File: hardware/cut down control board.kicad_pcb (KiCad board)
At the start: 2 copper layers, 42 parts, among them J1 CUTTER, J10 SAT(10 picoblade), J11 VGPS SELECT, J2 MOTOR, J3 AVR-ISP-6, J5 SAT(PIN HDR), J6 GPS(PIN HDR), J7 DBG TTL, J9 GPS(JST SH), Q1 FQP30N06L, Q2 FQP30N06L, U1 ATmega328-P, U2 MPL3115A2, U5 L78L33_TO92, U6 L7805, Y1 16MHz

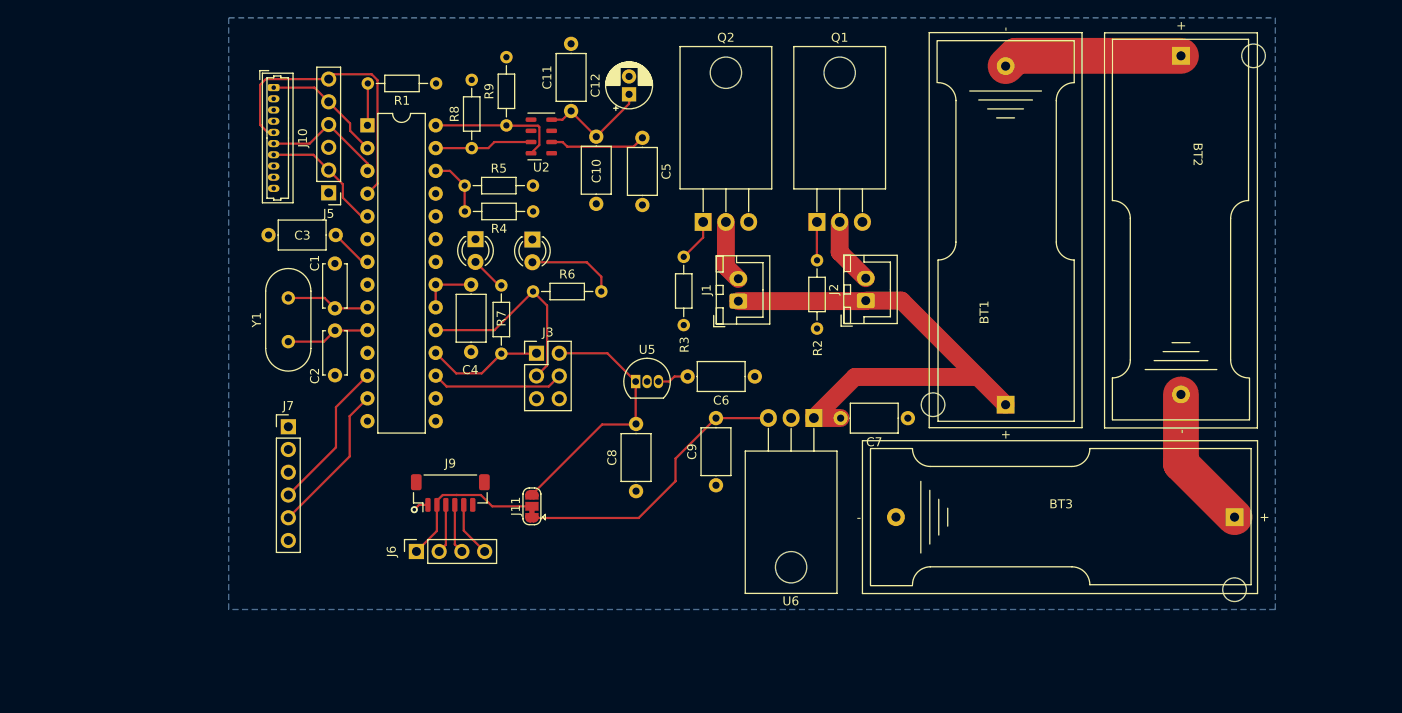
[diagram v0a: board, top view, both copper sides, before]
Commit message: finished board, generated gerbers
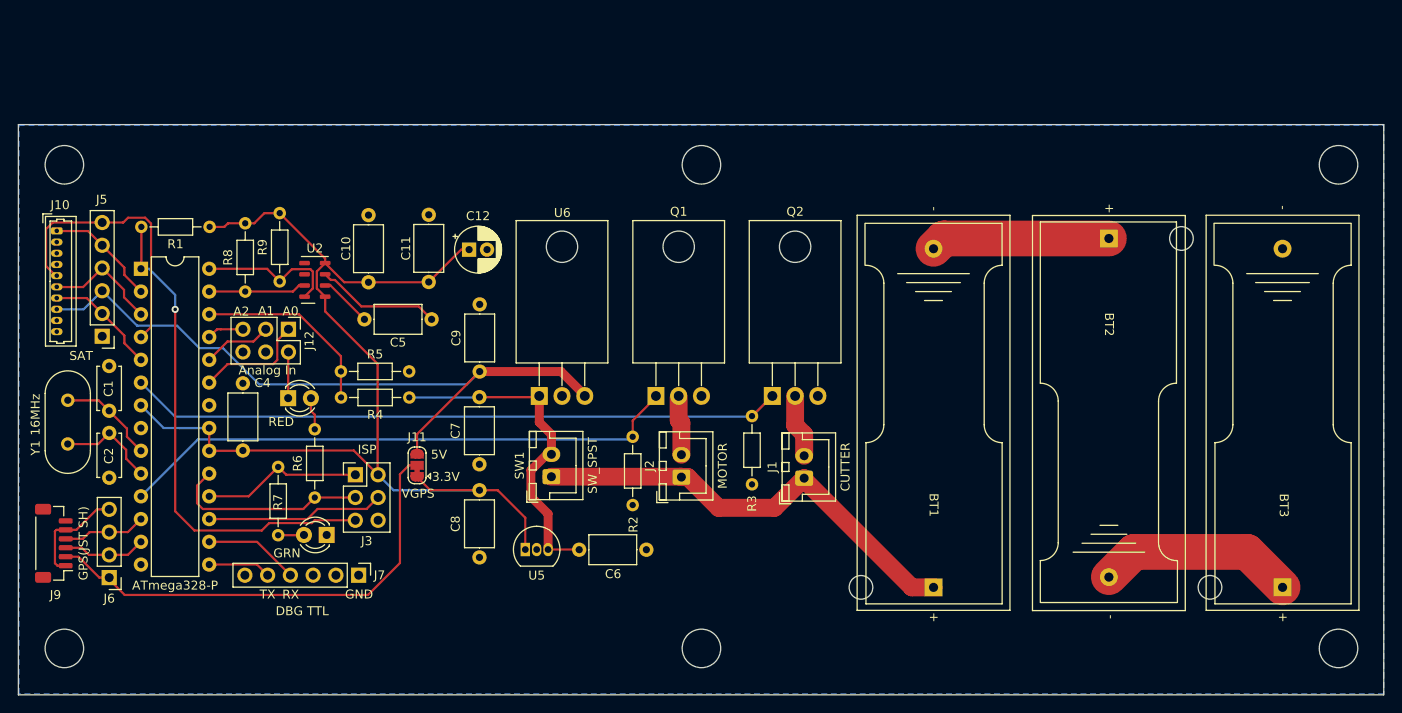
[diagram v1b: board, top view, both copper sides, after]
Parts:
- removed C3: 100nF, Capacitor_THT:C_Axial_L5.1mm_D3.1mm_P7.50mm_Horizontal
- added ?: , , F.Cu at (151.8, 126.3)
- added ?: , , F.Cu at (80.7, 72.3)
- added ?: , , F.Cu at (80.7, 126.3)
- added ?: , , F.Cu at (151.8, 72.3)
- added ?: , , F.Cu at (223.0, 126.3)
- added ?: , , F.Cu at (223.0, 72.3)
- added J12: Analog In, Connector_PinHeader_2.54mm:PinHeader_2x03_P2.54mm_Vertical, F.Cu at (105.7, 90.6)
- added SW1: SW_SPST, Connector_JST:JST_XH_B2B-XH-A_1x02_P2.50mm_Vertical, F.Cu at (135.1, 107.1)
- J3: value AVR-ISP-6 -> ISP
- J6: footprint Connector_PinSocket_2.54mm:PinSocket_1x04_P2.54mm_Vertical -> Connector_PinHeader_2.54mm:PinHeader_1x04_P2.54mm_Vertical
- moved C7 48.1 mm to (127.1, 105.7), turned to 90 degrees
- moved J9 44.6 mm to (79.5, 114.5), turned to 90 degrees
- moved C5 37.1 mm to (114.2, 89.5), turned to 0 degrees
- moved D2 37.0 mm to (110.0, 113.6), turned to 180 degrees
- moved J6 34.4 mm to (85.7, 118.4), turned to 180 degrees
- moved R6 33.5 mm to (108.7, 109.4), turned to 90 degrees
- moved C9 33.2 mm to (127.1, 87.9), turned to -90 degrees
- moved D1 32.5 mm to (105.7, 98.3), turned to 0 degrees
- moved C4 31.5 mm to (100.6, 104.2), turned to 90 degrees
- moved U6 30.8 mm to (133.7, 98.1), turned to 0 degrees
- moved R9 30.7 mm to (104.8, 85.3)
- moved C10 30.2 mm to (114.7, 85.4), turned to 90 degrees
- moved U2 29.9 mm to (108.7, 85.1)
- moved R1 29.9 mm to (96.9, 79.2)
- moved J5 29.9 mm to (84.9, 91.4)
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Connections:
- BT1 pad 1: +9V -> VDD
- J1 pad 1: +9V -> VDD
- J11 pad 1: +5V -> +3.3V
- J11 pad 3: +3.3V -> +5V
- J2 pad 1: +9V -> VDD
- U1 pad 12: /RX_DBG -> /RX_GPS
- U1 pad 13: /TX_DBG -> /TX_GPS
- U1 pad 15: /TX_GPS -> /TX_DBG
- U1 pad 16: /RX_GPS -> /RX_DBG
- U1 pad 23: unconnected-(U1-Pad23) -> /A0
- U1 pad 24: unconnected-(U1-Pad24) -> /A1
- U1 pad 25: unconnected-(U1-Pad25) -> /A2
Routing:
- net /CUTTER: track 4.79 -> 76.0 mm
- net +3.3V: track 53.6 -> 122.2 mm
- net /LETDOWN_MOTOR: track 4.29 -> 63.1 mm
- net VDD: track 0.00 -> 50.8 mm
- net /RESET: track 4.70 -> 55.3 mm, vias 0 -> 1
- net +5V: track 32.9 -> 77.9 mm
- net /+VGPS: track 18.1 -> 52.9 mm
- net +9V: track 65.9 -> 37.6 mm
- net GND: track 7.91 -> 31.1 mm, vias 1 -> 0
- net /BATT_SENSE: track 6.81 -> 21.3 mm
- net /A0: track 0.00 -> 12.6 mm
- net /TX_DBG: track 17.0 -> 7.01 mm
- net /A1: track 0.00 -> 7.72 mm
- net /RX_DBG: track 17.0 -> 10.6 mm
- net Net-(D1-Pad2): track 10.0 -> 3.65 mm
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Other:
- board outline added: 152.4 x 63.7 mm
- board text added: "https://github.com/dwkennedy/ballooning 10/11/2022"
